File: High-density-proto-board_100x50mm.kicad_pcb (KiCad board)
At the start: 2 copper layers, 99.1 x 49.5 mm, 201 parts

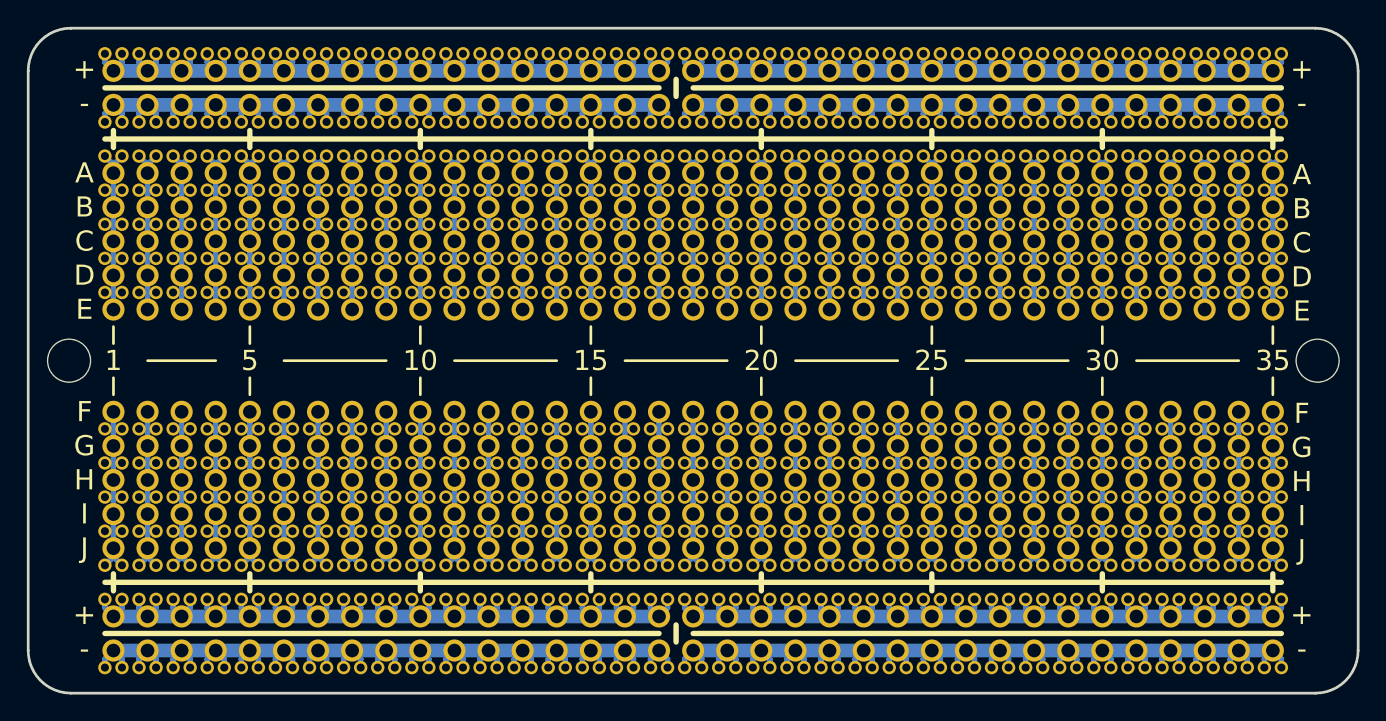
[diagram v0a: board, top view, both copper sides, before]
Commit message: Tweaks.
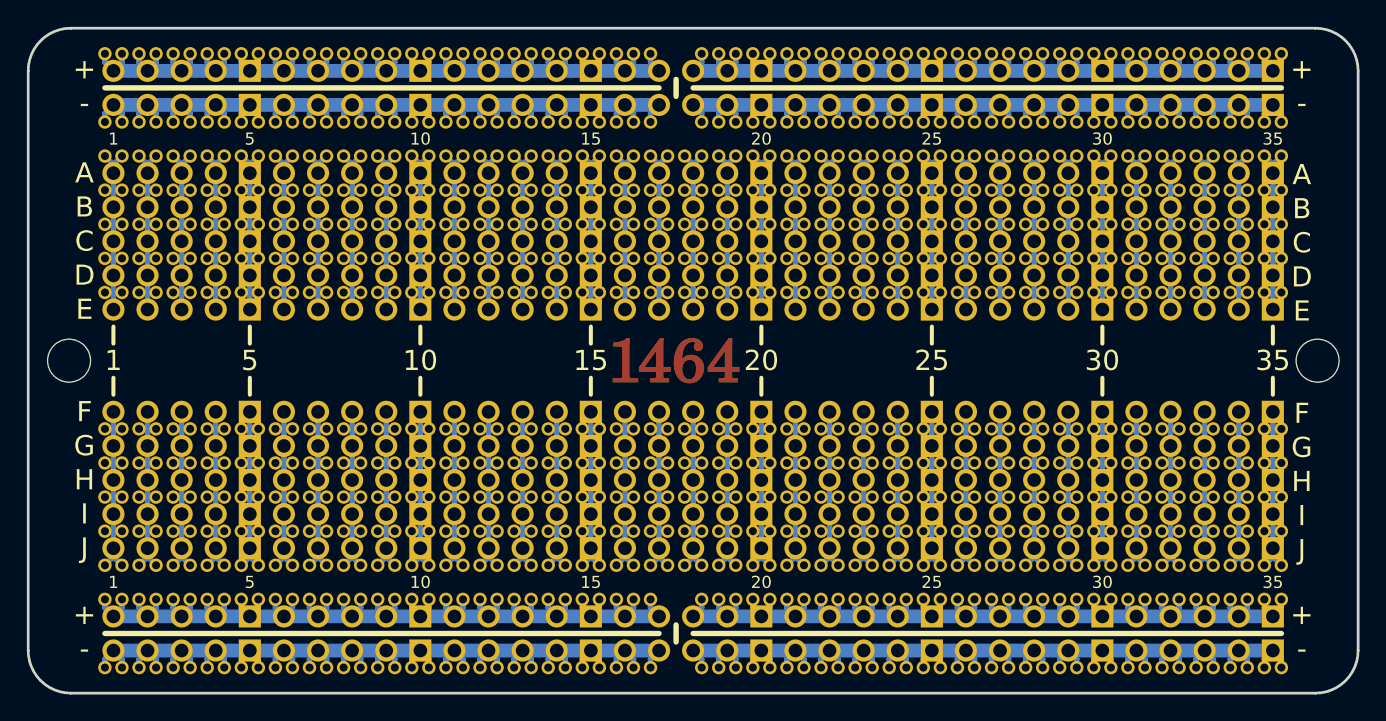
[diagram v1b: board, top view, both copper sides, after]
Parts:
- added G***: LOGO, LOGO, F.Cu at (69.2, 88.9)
- moved G*** 21.6 mm to (90.8, 88.9)
- moved G*** 19.0 mm to (47.6, 88.9)
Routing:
- net (no net): track 2011.7 -> 1999.4 mm
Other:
- board text added: "2014 - blog.spitzenpfeil.org 1464 - V0.10.a"
- board text removed: "2014 - blog.spitzenpfeil.org V0.10.a"
